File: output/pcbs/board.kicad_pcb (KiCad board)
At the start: 2 copper layers, 94 x 82 mm, 35 parts

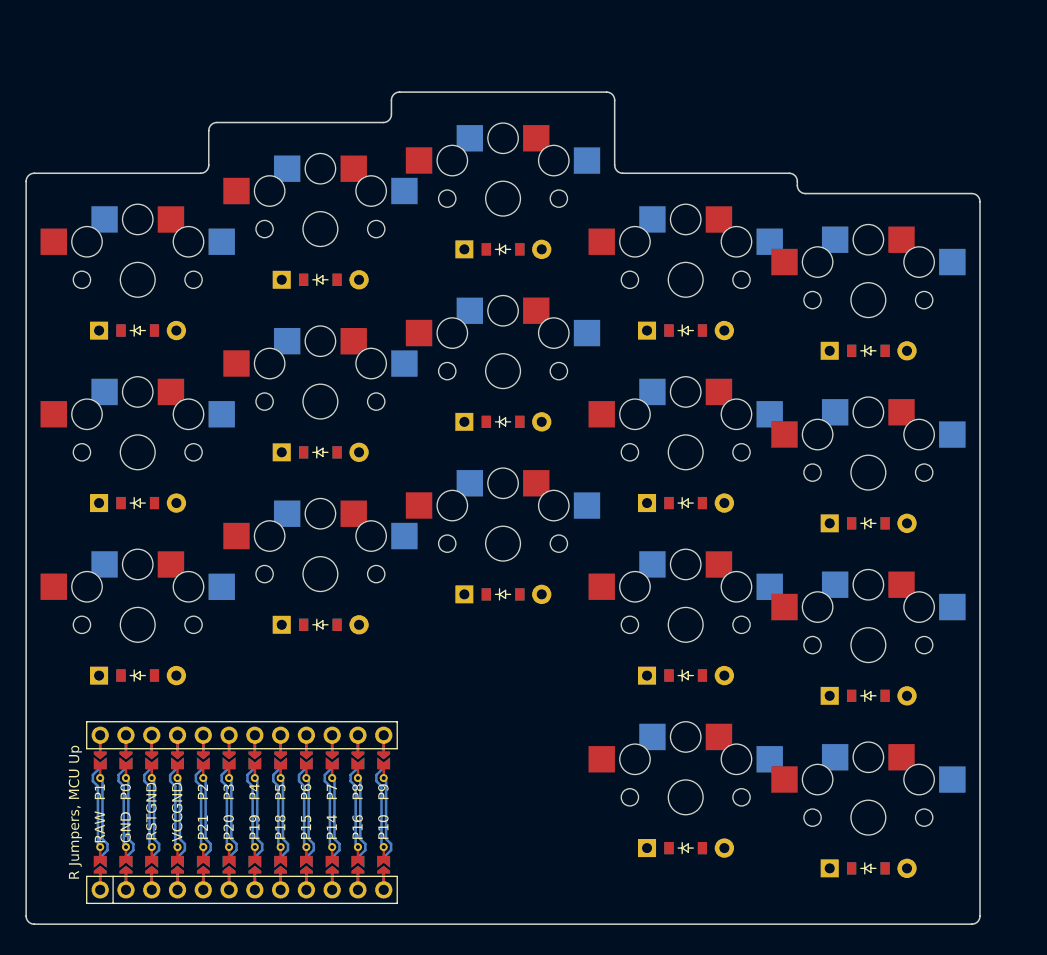
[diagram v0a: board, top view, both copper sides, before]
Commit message: final
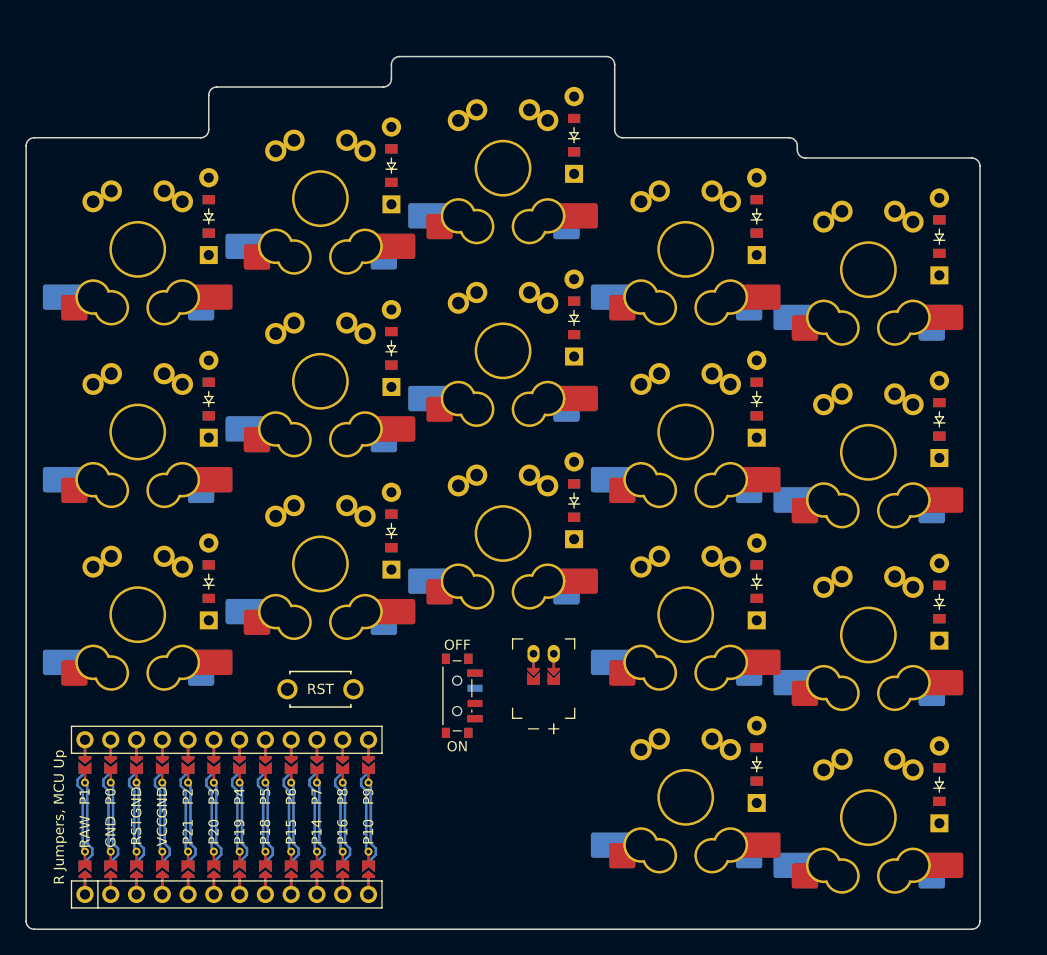
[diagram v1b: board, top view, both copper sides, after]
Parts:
- added JST1: , ceoloide:battery_connector_jst_ph_2, F.Cu at (215.0, 160.8)
- added PWR1: , ceoloide:power_switch_smd_side, F.Cu at (206.5, 165.0)
- added RST1: , ceoloide:reset_switch_tht_top, F.Cu at (193.0, 164.3)
- D1, D10, D11, D12, D13, D14, D15, D16, D17, D2, D3, D4, D5, D6, D7, D8, D9: footprint ComboDiode -> ceoloide:diode_tht_sod123; moved to B.Cu
- S1, S10, S11, S12, S13, S14, S15, S16, S17, S2, S3, S4, S5, S6, S7, S8, S9: footprint PG1350 -> ceoloide:switch_gateron_ks27_ks33; moved to B.Cu
- moved D13 13.2 mm to (236.0, 117.8), turned to 90 degrees
- moved D17 13.2 mm to (254.0, 119.8), turned to 90 degrees
- moved D3 13.2 mm to (182.0, 117.8), turned to 90 degrees
- moved D6 13.2 mm to (200.0, 112.8), turned to 90 degrees
- moved D9 13.2 mm to (218.0, 109.8), turned to 90 degrees
- moved D12 12.4 mm to (236.0, 135.8), turned to 90 degrees
- moved D16 12.4 mm to (254.0, 137.8), turned to 90 degrees
- moved D2 12.4 mm to (182.0, 135.8), turned to 90 degrees
- moved D5 12.4 mm to (200.0, 130.8), turned to 90 degrees
- moved D8 12.4 mm to (218.0, 127.8), turned to 90 degrees
- moved D1 11.6 mm to (182.0, 153.8), turned to 90 degrees
- moved D11 11.6 mm to (236.0, 153.8), turned to 90 degrees
- moved D15 11.6 mm to (254.0, 155.8), turned to 90 degrees
- moved D4 11.6 mm to (200.0, 148.8), turned to 90 degrees
- moved D7 11.6 mm to (218.0, 145.8), turned to 90 degrees
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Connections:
- D1 pad 1: P100 -> P14
- D10 pad 1: P024 -> P15
- D11 pad 1: P100 -> P14
- D12 pad 1: P011 -> P16
- D13 pad 1: P104 -> P10
- D14 pad 1: P024 -> P15
- D15 pad 1: P100 -> P14
- D16 pad 1: P011 -> P16
- D17 pad 1: P104 -> P10
- D2 pad 1: P011 -> P16
- D3 pad 1: P104 -> P10
- D4 pad 1: P100 -> P14
- D5 pad 1: P011 -> P16
- D6 pad 1: P104 -> P10
- D7 pad 1: P100 -> P14
- D8 pad 1: P011 -> P16
- D9 pad 1: P104 -> P10
- S1 pad : (no net) -> pinky_bottom
- S1 pad 1: P006 -> P2
- S10 pad : (no net) -> index_thumb
- S10 pad 1: P020 -> P5
- S11 pad : (no net) -> index_bottom
- S11 pad 1: P020 -> P5
- S12 pad : (no net) -> index_home
- S12 pad 1: P020 -> P5
- S13 pad : (no net) -> index_top
- S13 pad 1: P020 -> P5
- S14 pad : (no net) -> inner_thumb
- S14 pad 1: P022 -> P6
- S15 pad : (no net) -> inner_bottom
- S15 pad 1: P022 -> P6
- S16 pad : (no net) -> inner_home
- S16 pad 1: P022 -> P6
- S17 pad : (no net) -> inner_top
- S17 pad 1: P022 -> P6
- S2 pad : (no net) -> pinky_home
- S2 pad 1: P006 -> P2
- S3 pad : (no net) -> pinky_top
- S3 pad 1: P006 -> P2
- S4 pad : (no net) -> ring_bottom
- S4 pad 1: P008 -> P3
- S5 pad : (no net) -> ring_home
- S5 pad 1: P008 -> P3
- S6 pad : (no net) -> ring_top
- S6 pad 1: P008 -> P3
- S7 pad : (no net) -> middle_bottom
- S7 pad 1: P017 -> P4
- S8 pad : (no net) -> middle_home
- S8 pad 1: P017 -> P4
- S9 pad : (no net) -> middle_top
- S9 pad 1: P017 -> P4
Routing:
- net JST1_2: track 0.00 -> 3.60 mm
- net JST1_1: track 0.00 -> 3.60 mm
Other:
- board size 94 x 82 mm -> 94 x 86 mm

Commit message: padding adjust
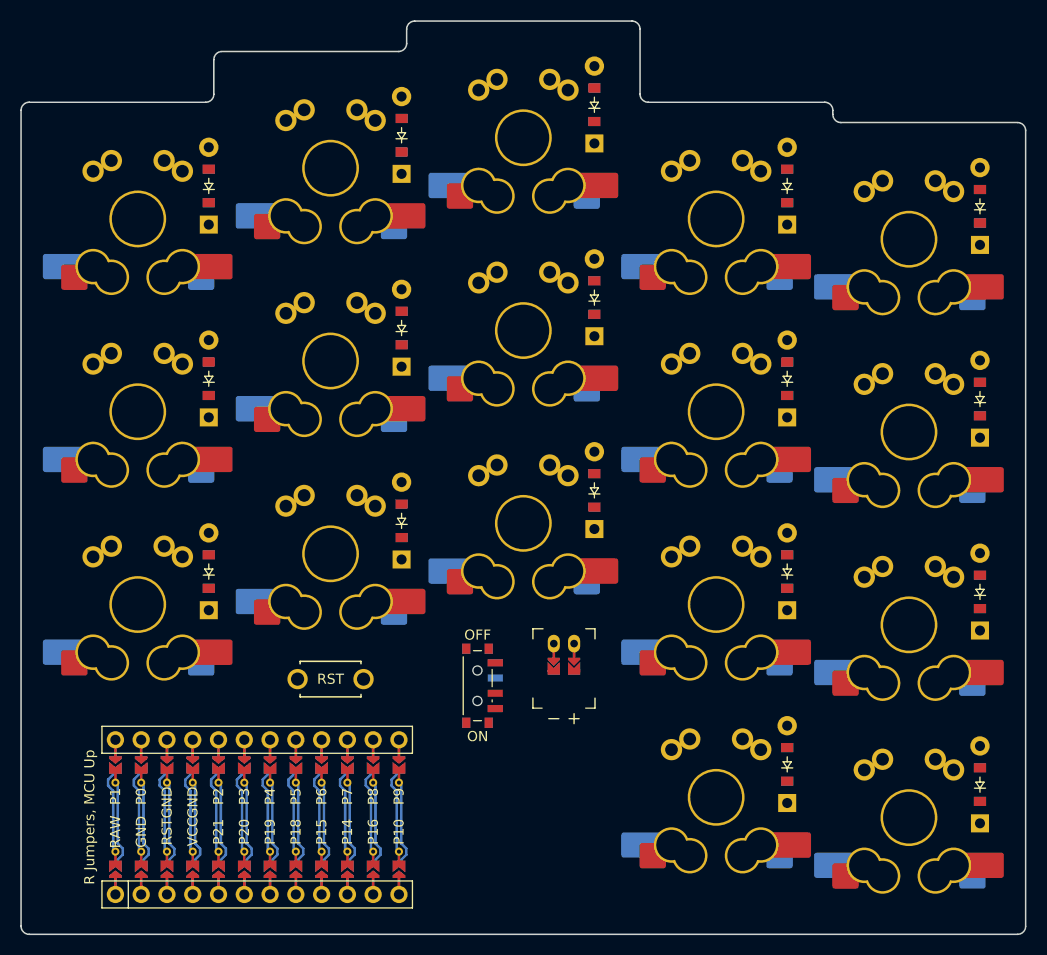
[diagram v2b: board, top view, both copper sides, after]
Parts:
- moved D17 5.00 mm to (258.0, 116.8)
- moved S17 5.00 mm to (251.0, 120.0)
- moved D16 4.47 mm to (258.0, 135.8)
- moved S16 4.47 mm to (251.0, 139.0)
- moved D13 4.24 mm to (239.0, 114.8)
- moved S13 4.24 mm to (232.0, 118.0)
- moved D15 4.12 mm to (258.0, 154.8)
- moved S15 4.12 mm to (251.0, 158.0)
- moved D14 4.00 mm to (258.0, 173.8)
- moved S14 4.00 mm to (251.0, 177.0)
- moved D12 3.61 mm to (239.0, 133.8)
- moved D9 3.61 mm to (220.0, 106.8)
- moved S12 3.61 mm to (232.0, 137.0)
- moved S9 3.61 mm to (213.0, 110.0)
- moved D11 3.16 mm to (239.0, 152.8)
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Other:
- board size 94 x 86 mm -> 99 x 90 mm
